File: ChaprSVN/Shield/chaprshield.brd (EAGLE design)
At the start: 72.7 x 47 mm, 16 parts, among them M2 RN42 Module

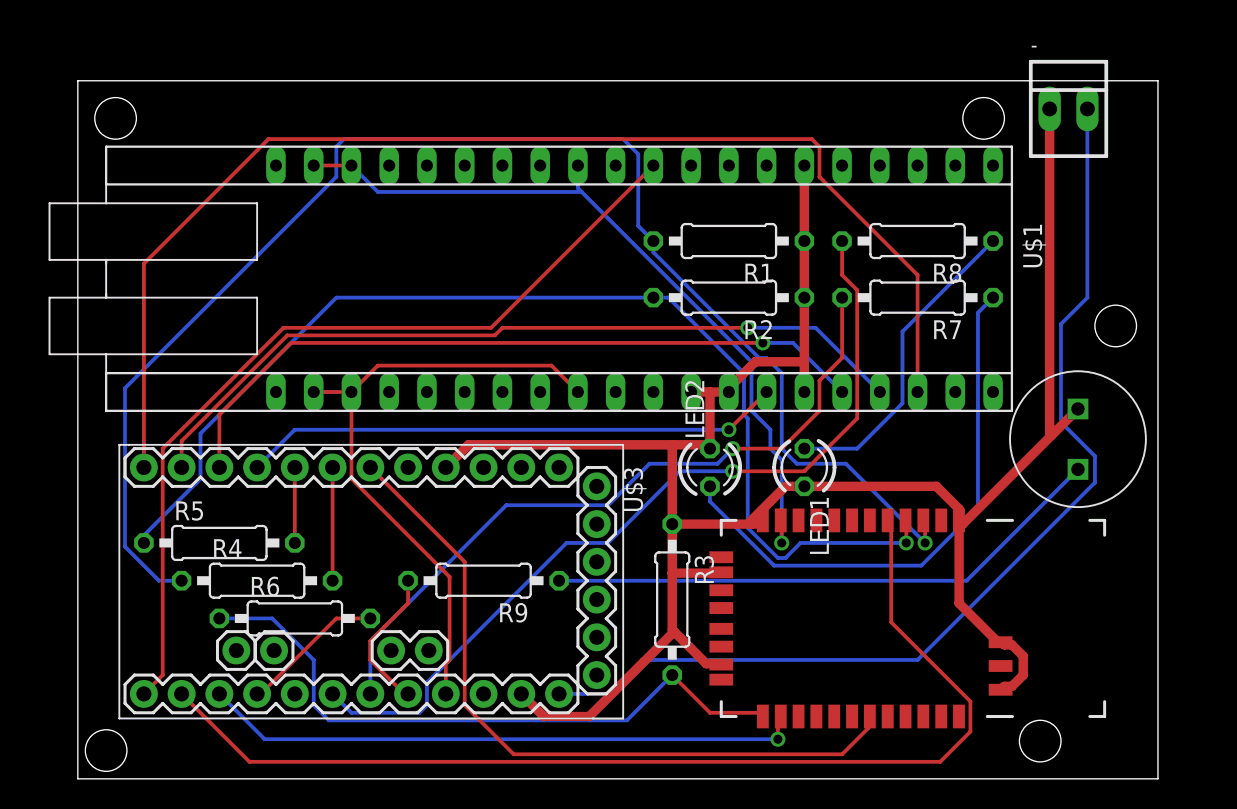
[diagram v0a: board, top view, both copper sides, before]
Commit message: First version of the ChapR board v0.2.  These files were sent to Sunstone.
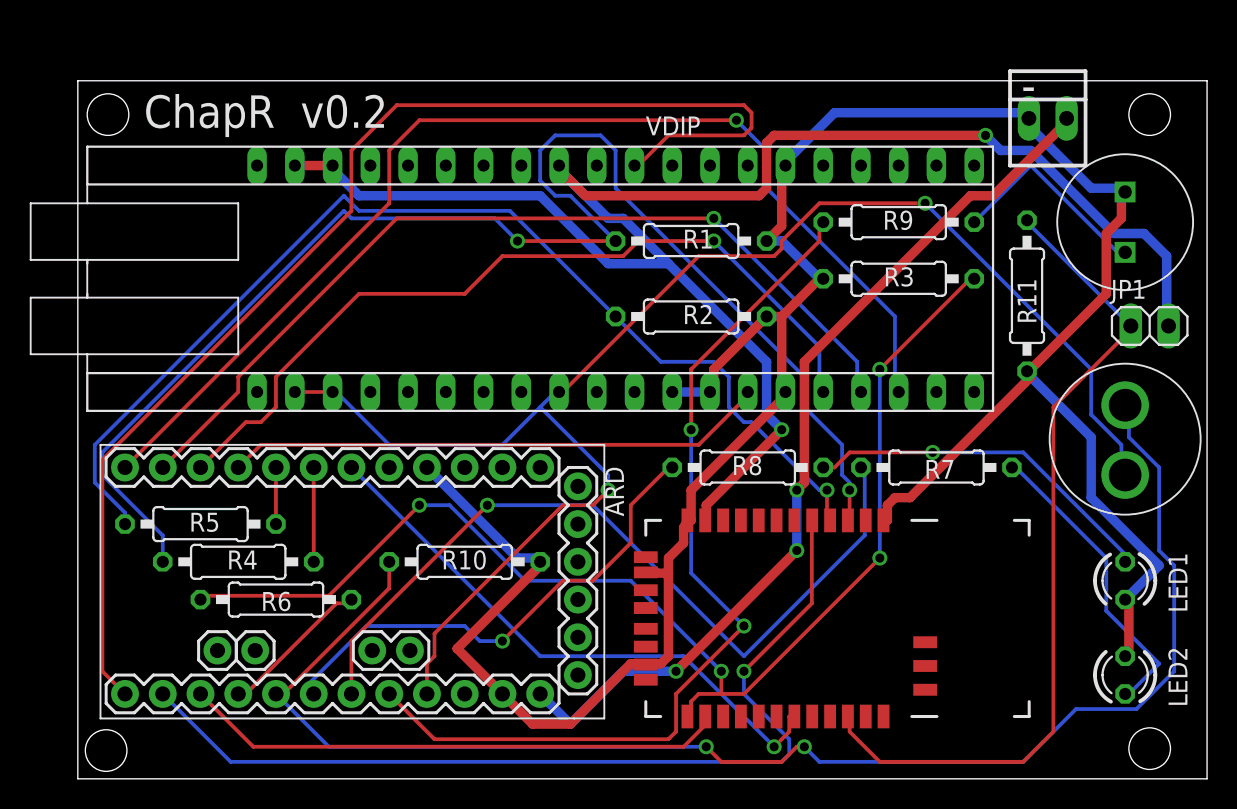
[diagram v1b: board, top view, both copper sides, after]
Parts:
- removed U$1: VDIP2, ChapR-Custom:VDIP2
- removed U$3: PROMINI, ChapR-Custom:PROMINI
- added ARD: PROMINI, ChapR-Custom:PROMINI
- added JP1: (no value), pinhead:1X02
- added PB1: PUSHBUTTON, ChapR-Custom:2-PIN-PUSHBUTTON
- added R10, R11: 10k, resistor:0207/10
- added VDIP: VDIP2, ChapR-Custom:VDIP2
- moved R9 36.9 mm to (54.6, 36.8)
- moved LED2 31.2 mm to (69.8, 6.35)
- moved R3 26.4 mm to (54.6, 33.0), turned to 0 degrees
- moved LED1 22.9 mm to (69.8, 12.7)
- moved R8 19.1 mm to (44.5, 20.3)
- moved U$2 14.9 mm to (69.8, 36.8)
- moved R7 11.5 mm to (57.1, 20.3)
- moved M2 5.08 mm to (47.0, 10.2)
- moved R2 2.84 mm to (40.6, 30.5)
- moved R1 2.54 mm to (40.6, 35.6)
- moved R5 1.80 mm to (7.62, 16.5)
- moved R4 1.80 mm to (10.2, 14.0)
- moved R6 1.80 mm to (12.7, 11.4)
- moved - 1.53 mm to (64.6, 43.8)
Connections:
- new net N$22: JP1.1, M2.22, R11.2
- new net N$24: ARD.A0, PB1.P$2, R10.2
- net +9V: now also ARD.RAWV; no longer U$3.RAWV
- net 3.3V: now also JP1.2, VDIP.32, VDIP.38, VDIP.39; no longer U$1.32, U$1.38, U$1.39
- net GND: now also ARD.GND, ARD.GND2, R10.1, R11.1, VDIP.12, VDIP.13, VDIP.15, VDIP.26; no longer M2.25, M2.27, U$1.12, U$1.13, U$1.15, U$1.26, U$3.GND, U$3.GND2
- net LED1(BD5): now also VDIP.4; no longer U$1.4
- net LED2(BD6): now also VDIP.5; no longer U$1.5
- net N$1: now also ARD.VCC, PB1.P$1, VDIP.2, VDIP.3, VDIP.9; no longer U$1.2, U$1.3, U$1.9, U$3.VCC
- net N$10: now also ARD.D9, VDIP.18; no longer U$1.18, U$3.D9
- net N$11: now also ARD.D8, VDIP.17; no longer U$1.17, U$3.D8
- net N$12: now also ARD.D7, VDIP.16; no longer U$1.16, U$3.D7
- net N$13: now also ARD.D6, VDIP.14; no longer U$1.14, U$3.D6
- net N$14: now also ARD.D4; no longer U$3.D4
- net N$15: now also ARD.D3; no longer U$3.D3
- net N$18: now also ARD.A2; no longer U$3.A2
- net N$2: now also ARD.D10, VDIP.30; no longer U$1.30, U$3.D10
- net N$20: now also ARD.A1; no longer U$3.A1
- net N$21: now also ARD.A3; no longer U$3.A3
- net N$3: now also ARD.D13; no longer U$3.D13
- net N$4: now also ARD.D12; no longer U$3.D12
- net N$5: now also ARD.D11; no longer U$3.D11
- net N$8: now also ARD.D5; no longer U$3.D5
- net NC(1): now also VDIP.1; no longer U$1.1
- net NC(2): now also VDIP.40; no longer U$1.40
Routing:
- net N$24: track 0.00 -> 97.4 mm, vias 0 -> 2
- net 3.3V: track 51.4 -> 115.2 mm, vias 1 -> 2
- net N$1: track 42.4 -> 102.4 mm, vias 0 -> 2
- net N$22: track 0.00 -> 55.9 mm
- net N$21: track 9.87 -> 62.1 mm, vias 0 -> 2
- net N$9: track 43.8 -> 83.3 mm, vias 0 -> 4
- net N$2: track 57.9 -> 82.5 mm
- net N$19: track 38.0 -> 14.4 mm
- net N$20: track 57.3 -> 33.8 mm
- net GND: track 150.3 -> 171.8 mm
- net N$16: track 37.1 -> 20.6 mm
- net N$15: track 48.8 -> 39.0 mm, vias 0 -> 1
- net N$5: track 72.3 -> 63.2 mm, vias 0 -> 1
- net +9V: track 68.8 -> 60.6 mm, vias 0 -> 3
- net N$11: track 53.7 -> 60.6 mm
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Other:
- board size 72.7 x 47 mm -> 76 x 47 mm
- board text added: "ChapR v0.2"
